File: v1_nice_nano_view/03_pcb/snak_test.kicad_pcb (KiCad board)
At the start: 2 copper layers, 114.1 x 99.4 mm, 99 parts

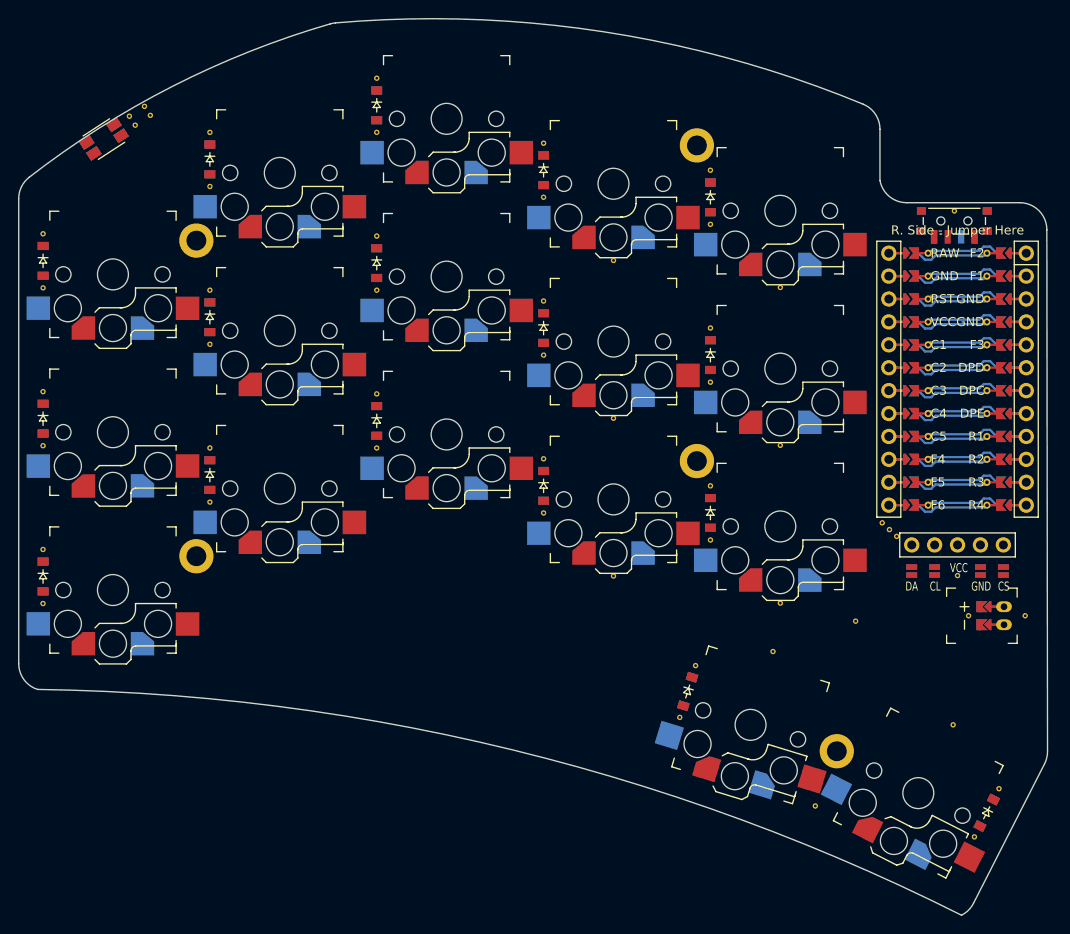
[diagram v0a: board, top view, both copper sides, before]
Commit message: update
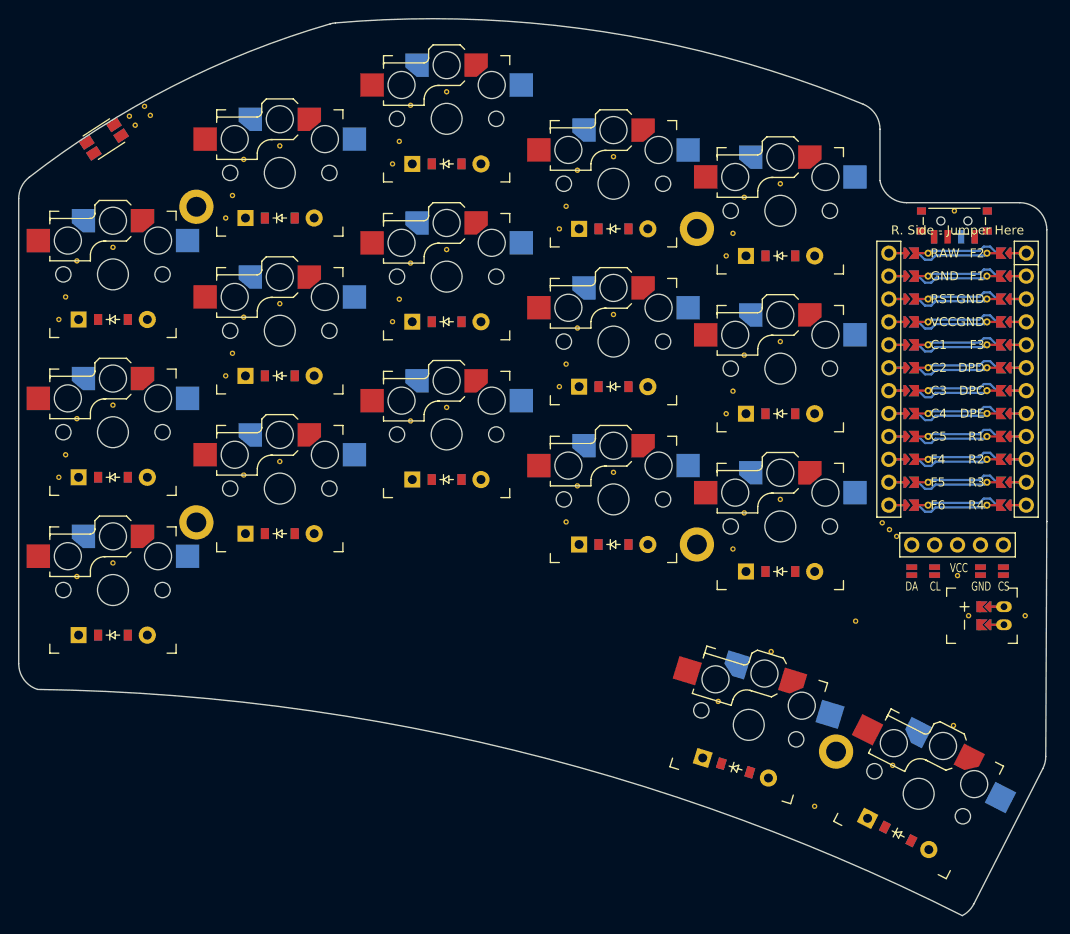
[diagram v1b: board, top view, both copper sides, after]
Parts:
- removed the REF** at (92.2, 95.5)
- removed the REF** at (147.8, 85.5)
- removed the REF** at (147.8, 68.0)
- removed the REF** at (147.8, 50.5)
- removed the REF** at (166.2, 88.5)
- removed the REF** at (166.2, 71.0)
- removed the REF** at (166.2, 53.5)
- removed the REF** at (164.6, 108.4)
- removed the REF** at (198.2, 122.0)
- removed the REF** at (92.2, 101.5)
- removed the REF** at (92.2, 84.0)
- removed the REF** at (92.2, 78.0)
- removed the REF** at (92.2, 66.5)
- removed the REF** at (110.8, 90.2)
- removed the REF** at (110.8, 72.8)
- removed the REF** at (110.8, 55.2)
- removed the REF** at (129.2, 84.2)
- removed the REF** at (129.2, 66.8)
- removed the REF** at (129.2, 49.2)
- removed the REF** at (147.8, 91.5)
- removed the REF** at (147.8, 74.0)
- removed the REF** at (147.8, 56.5)
- removed the REF** at (92.2, 60.5)
- removed the REF** at (166.2, 94.5)
- removed the REF** at (166.2, 77.0)
- removed the REF** at (166.2, 59.5)
- removed the REF** at (162.9, 114.1)
- removed the REF** at (195.5, 127.4)
- removed the REF** at (155.5, 98.5)
- removed the REF** at (155.5, 81.0)
- removed the REF** at (155.5, 63.5)
- removed the REF** at (174.0, 101.5)
- removed the REF** at (174.0, 84.0)
- removed the REF** at (110.8, 84.2)
- removed the REF** at (174.0, 66.5)
- removed the REF** at (177.9, 123.9)
- removed the REF** at (173.2, 106.8)
- removed the REF** at (193.2, 114.9)
- removed the REF** at (110.8, 66.8)
- removed the REF** at (110.8, 49.2)
- removed the REF** at (129.2, 78.2)
- removed the REF** at (129.2, 60.8)
- removed the REF** at (129.2, 43.2)
- added REF**: VIA-0.6mm, VIA-0.6mm, F.Cu at (96.0, 98.5)
- added REF**: VIA-0.6mm, VIA-0.6mm, F.Cu at (151.5, 88.5)
- added REF**: VIA-0.6mm, VIA-0.6mm, F.Cu at (151.5, 71.0)
- added REF**: VIA-0.6mm, VIA-0.6mm, F.Cu at (151.5, 53.5)
- added REF**: VIA-0.6mm, VIA-0.6mm, F.Cu at (170.0, 91.5)
- added REF**: VIA-0.6mm, VIA-0.6mm, F.Cu at (170.0, 74.0)
- added REF**: VIA-0.6mm, VIA-0.6mm, F.Cu at (170.0, 56.5)
- added REF**: VIA-0.6mm, VIA-0.6mm, F.Cu at (167.1, 112.3)
- added REF**: VIA-0.6mm, VIA-0.6mm, F.Cu at (186.5, 119.4)
- added REF**: VIA-0.6mm, VIA-0.6mm, F.Cu at (94.0, 87.5)
- added REF**: VIA-0.6mm, VIA-0.6mm, F.Cu at (94.0, 70.0)
- added REF**: VIA-0.6mm, VIA-0.6mm, F.Cu at (96.0, 81.0)
- added REF**: VIA-0.6mm, VIA-0.6mm, F.Cu at (112.5, 76.2)
- added REF**: VIA-0.6mm, VIA-0.6mm, F.Cu at (112.5, 58.8)
- added REF**: VIA-0.6mm, VIA-0.6mm, F.Cu at (131.0, 70.2)
- added REF**: VIA-0.6mm, VIA-0.6mm, F.Cu at (131.0, 52.8)
- added REF**: VIA-0.6mm, VIA-0.6mm, F.Cu at (149.5, 77.5)
- added REF**: VIA-0.6mm, VIA-0.6mm, F.Cu at (149.5, 60.0)
- added REF**: VIA-0.6mm, VIA-0.6mm, F.Cu at (168.0, 80.5)
- added REF**: VIA-0.6mm, VIA-0.6mm, F.Cu at (168.0, 63.0)
- added REF**: VIA-0.6mm, VIA-0.6mm, F.Cu at (100.0, 97.0)
- added REF**: VIA-0.6mm, VIA-0.6mm, F.Cu at (100.0, 79.5)
- added REF**: VIA-0.6mm, VIA-0.6mm, F.Cu at (96.0, 63.5)
- added REF**: VIA-0.6mm, VIA-0.6mm, F.Cu at (100.0, 62.0)
- added REF**: VIA-0.6mm, VIA-0.6mm, F.Cu at (118.5, 85.8)
- added REF**: VIA-0.6mm, VIA-0.6mm, F.Cu at (118.5, 68.2)
- added REF**: VIA-0.6mm, VIA-0.6mm, F.Cu at (118.5, 50.8)
- added REF**: VIA-0.6mm, VIA-0.6mm, F.Cu at (137.0, 79.8)
- added REF**: VIA-0.6mm, VIA-0.6mm, F.Cu at (137.0, 62.2)
- added REF**: VIA-0.6mm, VIA-0.6mm, F.Cu at (137.0, 44.8)
- added REF**: VIA-0.6mm, VIA-0.6mm, F.Cu at (155.5, 87.0)
- added REF**: VIA-0.6mm, VIA-0.6mm, F.Cu at (155.5, 69.5)
- added REF**: VIA-0.6mm, VIA-0.6mm, F.Cu at (155.5, 52.0)
- added REF**: VIA-0.6mm, VIA-0.6mm, F.Cu at (114.5, 87.2)
- added REF**: VIA-0.6mm, VIA-0.6mm, F.Cu at (174.0, 90.0)
- added REF**: VIA-0.6mm, VIA-0.6mm, F.Cu at (174.0, 72.5)
- added REF**: VIA-0.6mm, VIA-0.6mm, F.Cu at (174.0, 55.0)
- added REF**: VIA-0.6mm, VIA-0.6mm, F.Cu at (94.8, 85.0)
- added REF**: VIA-0.6mm, VIA-0.6mm, F.Cu at (94.8, 67.5)
- added REF**: VIA-0.6mm, VIA-0.6mm, F.Cu at (113.2, 73.8)
- added REF**: VIA-0.6mm, VIA-0.6mm, F.Cu at (113.2, 56.2)
- added REF**: VIA-0.6mm, VIA-0.6mm, F.Cu at (131.8, 67.8)
- added REF**: VIA-0.6mm, VIA-0.6mm, F.Cu at (131.8, 50.2)
- added REF**: VIA-0.6mm, VIA-0.6mm, F.Cu at (150.2, 92.5)
- added REF**: VIA-0.6mm, VIA-0.6mm, F.Cu at (114.5, 69.8)
- added REF**: VIA-0.6mm, VIA-0.6mm, F.Cu at (150.2, 75.0)
- added REF**: VIA-0.6mm, VIA-0.6mm, F.Cu at (150.2, 57.5)
- added REF**: VIA-0.6mm, VIA-0.6mm, F.Cu at (168.8, 95.5)
- added REF**: VIA-0.6mm, VIA-0.6mm, F.Cu at (168.8, 78.0)
- added REF**: VIA-0.6mm, VIA-0.6mm, F.Cu at (168.8, 60.5)
- added REF**: VIA-0.6mm, VIA-0.6mm, F.Cu at (177.8, 124.0)
- added REF**: VIA-0.6mm, VIA-0.6mm, F.Cu at (173.0, 106.8)
- added REF**: VIA-0.6mm, VIA-0.6mm, F.Cu at (193.2, 115.0)
- added REF**: VIA-0.6mm, VIA-0.6mm, F.Cu at (114.5, 52.2)
- added REF**: VIA-0.6mm, VIA-0.6mm, F.Cu at (133.0, 81.2)
- added REF**: VIA-0.6mm, VIA-0.6mm, F.Cu at (133.0, 63.8)
- added REF**: VIA-0.6mm, VIA-0.6mm, F.Cu at (133.0, 46.2)
- moved D1 10.1 mm to (100.0, 105.0), turned to 0 degrees
- moved D10 10.1 mm to (155.5, 95.0), turned to 0 degrees
- moved D11 10.1 mm to (155.5, 77.5), turned to 0 degrees
- moved D12 10.1 mm to (155.5, 60.0), turned to 0 degrees
- moved D13 10.1 mm to (174.0, 98.0), turned to 0 degrees
- moved D14 10.1 mm to (174.0, 80.5), turned to 0 degrees
- moved D15 10.1 mm to (174.0, 63.0), turned to 0 degrees
- moved D2 10.1 mm to (100.0, 87.5), turned to 0 degrees
- moved D3 10.1 mm to (100.0, 70.0), turned to 0 degrees
- moved D4 10.1 mm to (118.5, 93.8), turned to 0 degrees
- moved D5 10.1 mm to (118.5, 76.2), turned to 0 degrees
- moved D6 10.1 mm to (118.5, 58.8), turned to 0 degrees
- moved D7 10.1 mm to (137.0, 87.8), turned to 0 degrees
- moved D8 10.1 mm to (137.0, 70.2), turned to 0 degrees
- moved D9 10.1 mm to (137.0, 52.8), turned to 0 degrees
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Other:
- board size 114.1 x 99.4 mm -> 114 x 99.5 mm
